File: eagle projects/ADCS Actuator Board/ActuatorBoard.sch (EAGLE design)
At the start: 231 parts, among them J11 TE_1-84953-1, J2 TE_1-84953-1, J4 TE_1-84953-1, J5 TE-1734829-3, U10 LM2917MX/NOPB, U11 BD6210F-E2, U12 TSV991AILT, U13 LM2917MX/NOPB, U14 ADS7841E_2K5, U16 DRV10970_MOTOR_DRIVERDRV10970, U17 LM2917MX/NOPB, U18 BD6210F-E2, U19 TSV991AILT, U20 ADS7841E_2K5, U5 BD6210F-E2, U6 DRV10970_MOTOR_DRIVERDRV10970, U7 DRV10970_MOTOR_DRIVERDRV10970, U8 TSV991AILT, U9 ADS7841E_2K5

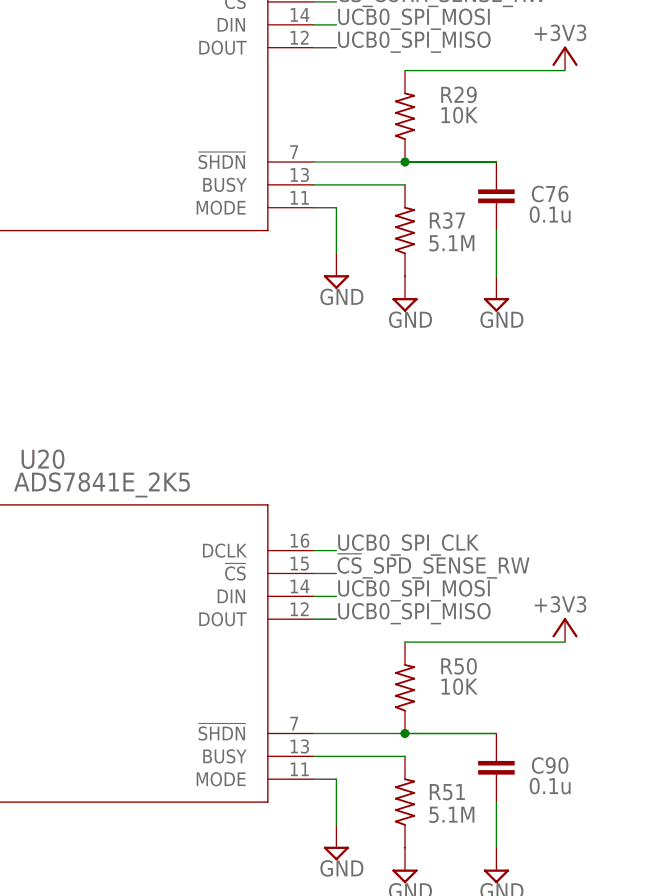
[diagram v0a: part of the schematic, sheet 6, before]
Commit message: Rev B almost ready
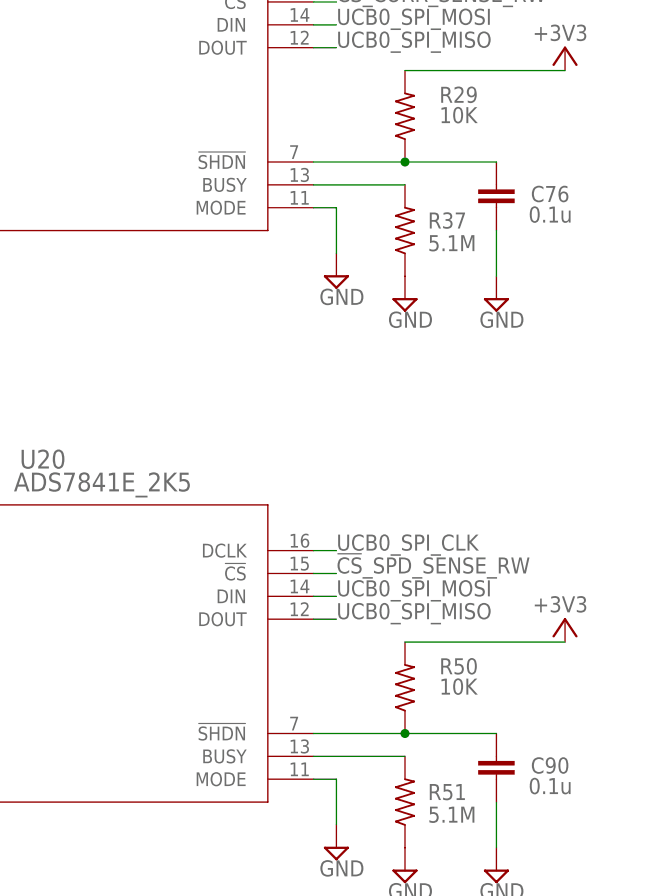
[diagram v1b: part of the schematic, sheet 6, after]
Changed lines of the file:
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@@
 </segment>
 </net>
-<net name="N$18" class="0">
-<segment>
-<pinref part="C69" gate="G$1" pin="1"/>
-<pinref part="R5" gate="G$1" pin="1"/>
-<pinref part="U9" gate="A" pin="!SHDN"/>
-<wire x1="149.86" y1="40.64" x2="129.54" y2="40.64" width="0.1524" layer="91"/>
-<junction x="139.7" y="40.64"/>
-<wire x1="149.86" y1="40.64" x2="139.7" y2="40.64" width="0.1524" layer="91"/>
-</segment>
-</net>
 <net name="N$25" class="0">
 <segment>
@@
 </segment>
 </net>
+<net name="N$2" class="0">
+<segment>
+<pinref part="U9" gate="A" pin="!SHDN"/>
+<pinref part="R5" gate="G$1" pin="1"/>
+<wire x1="129.54" y1="40.64" x2="139.7" y2="40.64" width="0.1524" layer="91"/>
+<pinref part="C69" gate="G$1" pin="1"/>
+<wire x1="139.7" y1="40.64" x2="149.86" y2="40.64" width="0.1524" layer="91"/>
+<junction x="139.7" y="40.64"/>
+</segment>
+</net>
 </nets>
 </sheet>
@@
 </segment>
 </net>
-<net name="N$33" class="0">
-<segment>
-<pinref part="C76" gate="G$1" pin="1"/>
-<pinref part="R29" gate="G$1" pin="1"/>
-<pinref part="U14" gate="A" pin="!SHDN"/>
-<wire x1="185.42" y1="152.4" x2="165.1" y2="152.4" width="0.1524" layer="91"/>
-<junction x="175.26" y="152.4"/>
-<wire x1="185.42" y1="152.4" x2="175.26" y2="152.4" width="0.1524" layer="91"/>
-</segment>
-</net>
 <net name="N$45" class="0">
 <segment>
@@
 </segment>
 </net>
-<net name="N$58" class="0">
-<segment>
-<pinref part="C90" gate="G$1" pin="1"/>
-<pinref part="R50" gate="G$1" pin="1"/>
-<pinref part="U20" gate="A" pin="!SHDN"/>
-<wire x1="185.42" y1="88.9" x2="165.1" y2="88.9" width="0.1524" layer="91"/>
-<junction x="175.26" y="88.9"/>
-<wire x1="185.42" y1="88.9" x2="175.26" y2="88.9" width="0.1524" layer="91"/>
-</segment>
-</net>
 <net name="N$59" class="0">
 <segment>
@@
 </segment>
 </net>
+<net name="N$4" class="0">
+<segment>
+<pinref part="U14" gate="A" pin="!SHDN"/>
+<pinref part="R29" gate="G$1" pin="1"/>
+<wire x1="165.1" y1="152.4" x2="175.26" y2="152.4" width="0.1524" layer="91"/>
+<pinref part="C76" gate="G$1" pin="1"/>
+<wire x1="175.26" y1="152.4" x2="185.42" y2="152.4" width="0.1524" layer="91"/>
+<junction x="175.26" y="152.4"/>
+</segment>
+</net>
+<net name="N$7" class="0">
+<segment>
+<pinref part="U20" gate="A" pin="!SHDN"/>
+<pinref part="R50" gate="G$1" pin="1"/>
+<wire x1="165.1" y1="88.9" x2="175.26" y2="88.9" width="0.1524" layer="91"/>
+<pinref part="C90" gate="G$1" pin="1"/>
+<wire x1="175.26" y1="88.9" x2="185.42" y2="88.9" width="0.1524" layer="91"/>
+<junction x="175.26" y="88.9"/>
+</segment>
+</net>
